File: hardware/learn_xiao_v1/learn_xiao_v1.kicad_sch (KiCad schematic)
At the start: 28 parts, among them J1 P0, J10 Conn_02x02_Odd_Even, J2 P1, J3 IO, J4 Conn_02x02_Odd_Even, J5 TYPE-C-31-M-12, J6 GY-87_10DOF, J7 Conn_02x08_Odd_Even, J8 Conn_02x05_Odd_Even, J9 Pot, SW1 SW_Push, SW2 SW_Push, U1 XIAO-SMD, U2 CH340N, U3 W25Q32JVSS, U4 OLED096, U5 LM35-LP

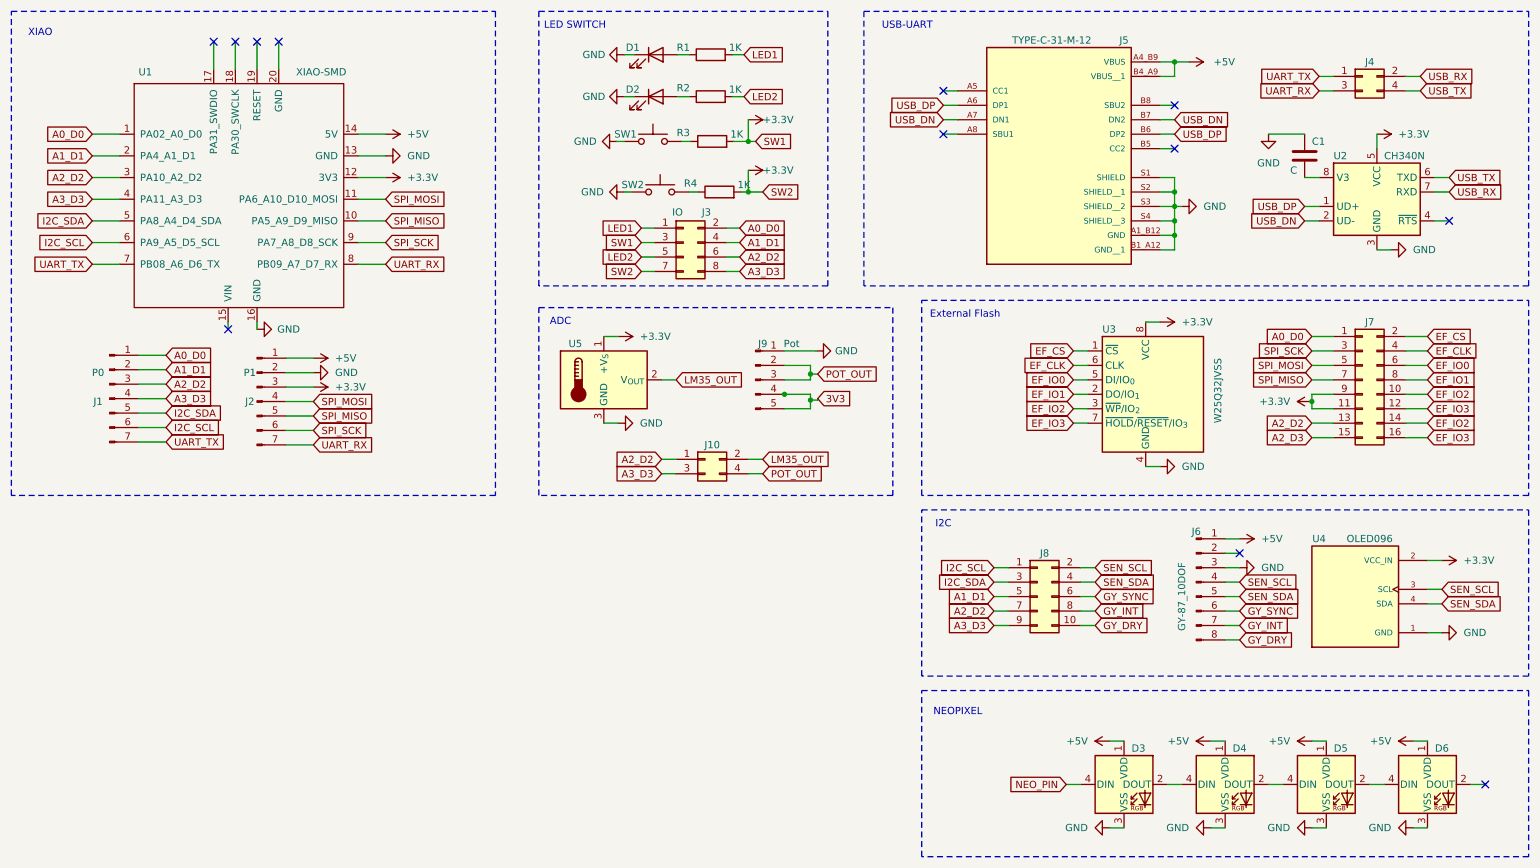
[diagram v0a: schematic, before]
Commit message: added webapp for pdm
added webapp for pdm
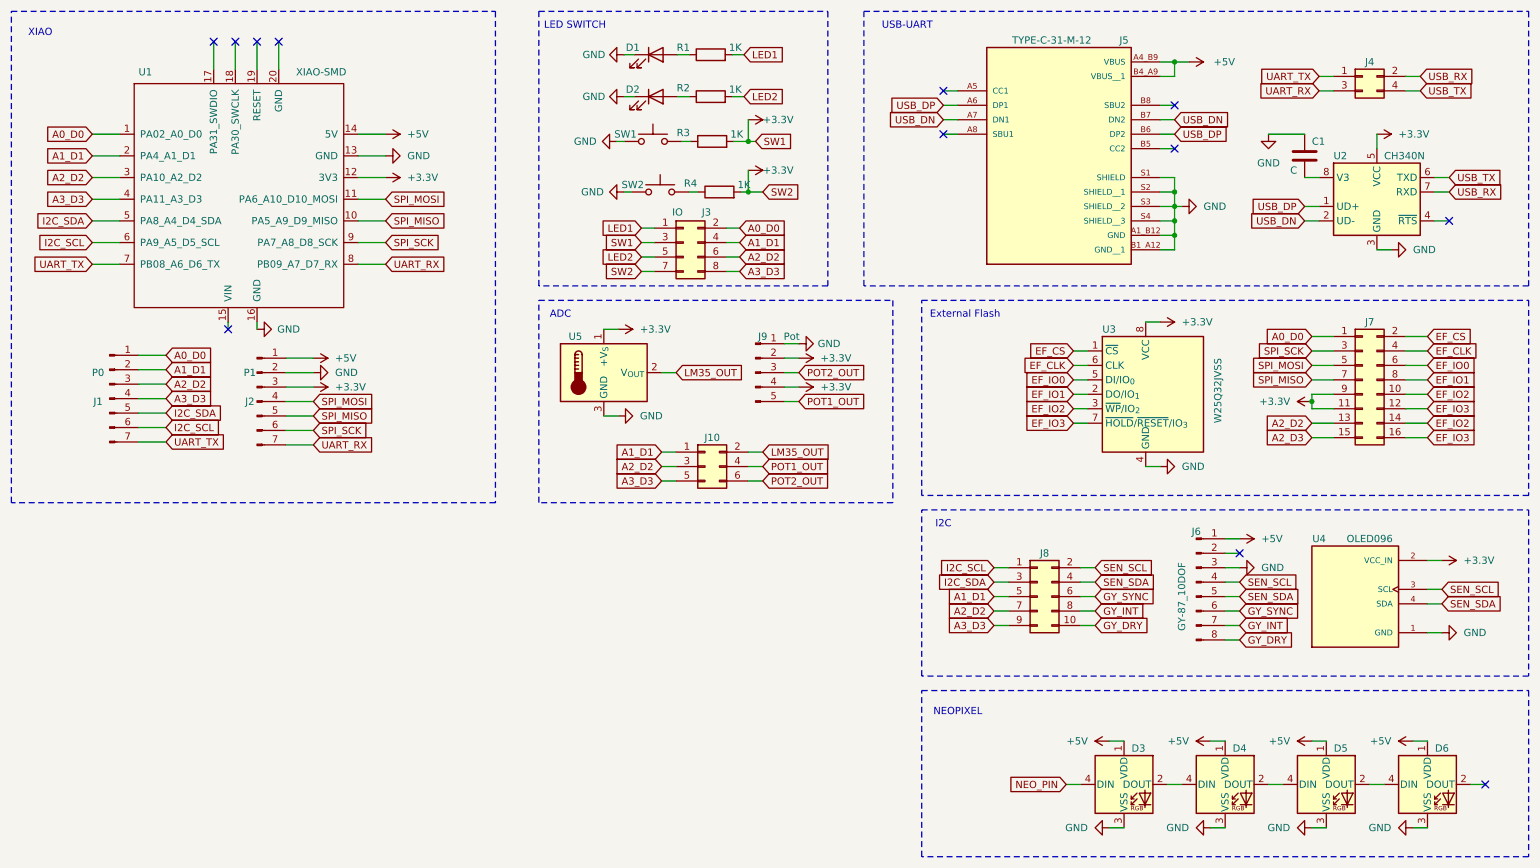
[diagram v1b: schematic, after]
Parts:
- removed J10: Conn_02x02_Odd_Even, symbol Connector_Generic:Conn_02x02_Odd_Even
- added J10: Conn_02x03_Odd_Even, symbol Connector_Generic:Conn_02x03_Odd_Even
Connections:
- net +3.3V: now also J9.2 (Pin_2), J9.4 (Pin_4)
- net A1_D1: now also J10.1 (Pin_1)
- net A2_D2: now also J10.3 (Pin_3)
- net A3_D3: now also J10.5 (Pin_5)
- net LM35_OUT: now also J10.2 (Pin_2)
- net 3V3 renamed POT1_OUT
- net POT1_OUT: now also J10.4 (Pin_4); no longer J9.4 (Pin_4)
- net POT_OUT renamed POT2_OUT
- net POT2_OUT: now also J10.6 (Pin_6); no longer J9.2 (Pin_2)
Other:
- moved on the sheet: J9, U5
